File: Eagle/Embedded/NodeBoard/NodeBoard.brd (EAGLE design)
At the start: 121.7 x 96 mm, 68 parts, among them IC1 7812TV, IC2 5v, IC3 3v3, IC4 REG1117, IC5 REG1117, J1 DCJ0202, Q2 IRF740, T1 BC547

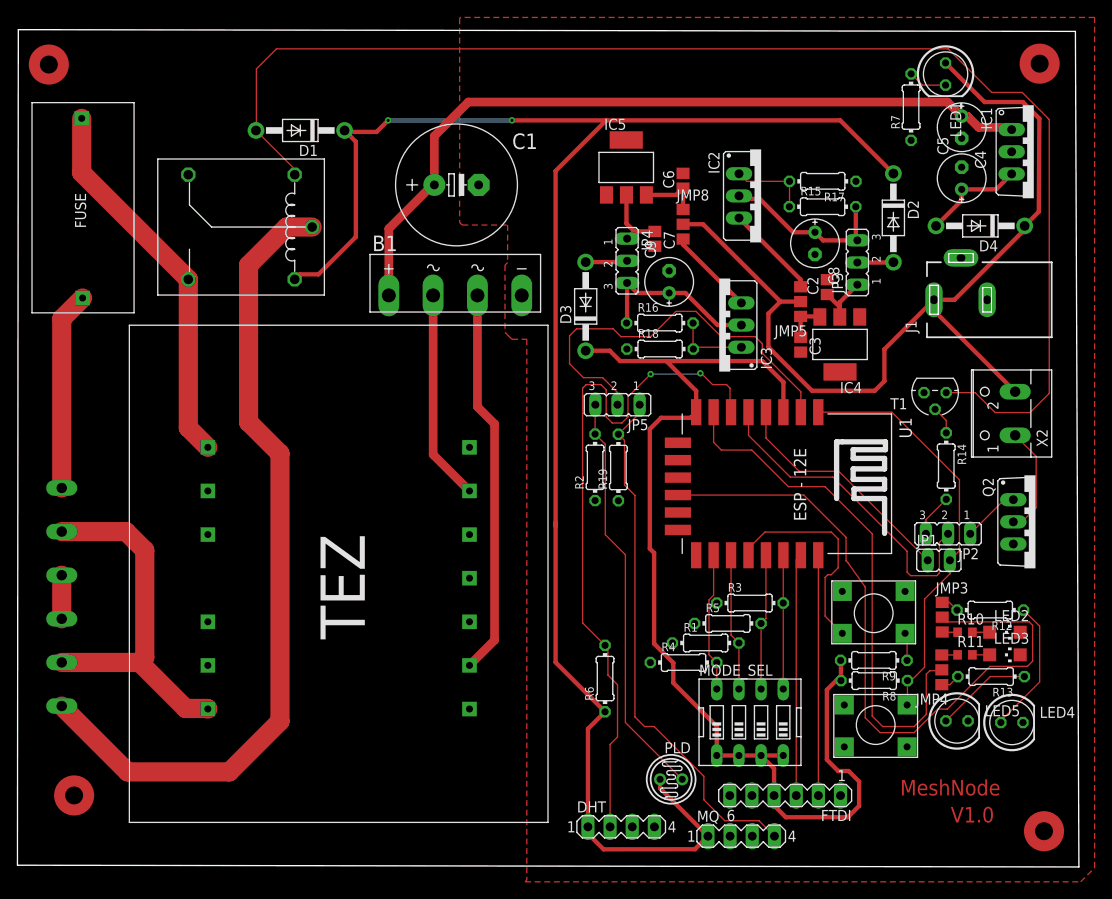
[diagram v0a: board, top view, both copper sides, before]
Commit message: Minor Eagle Board fixes
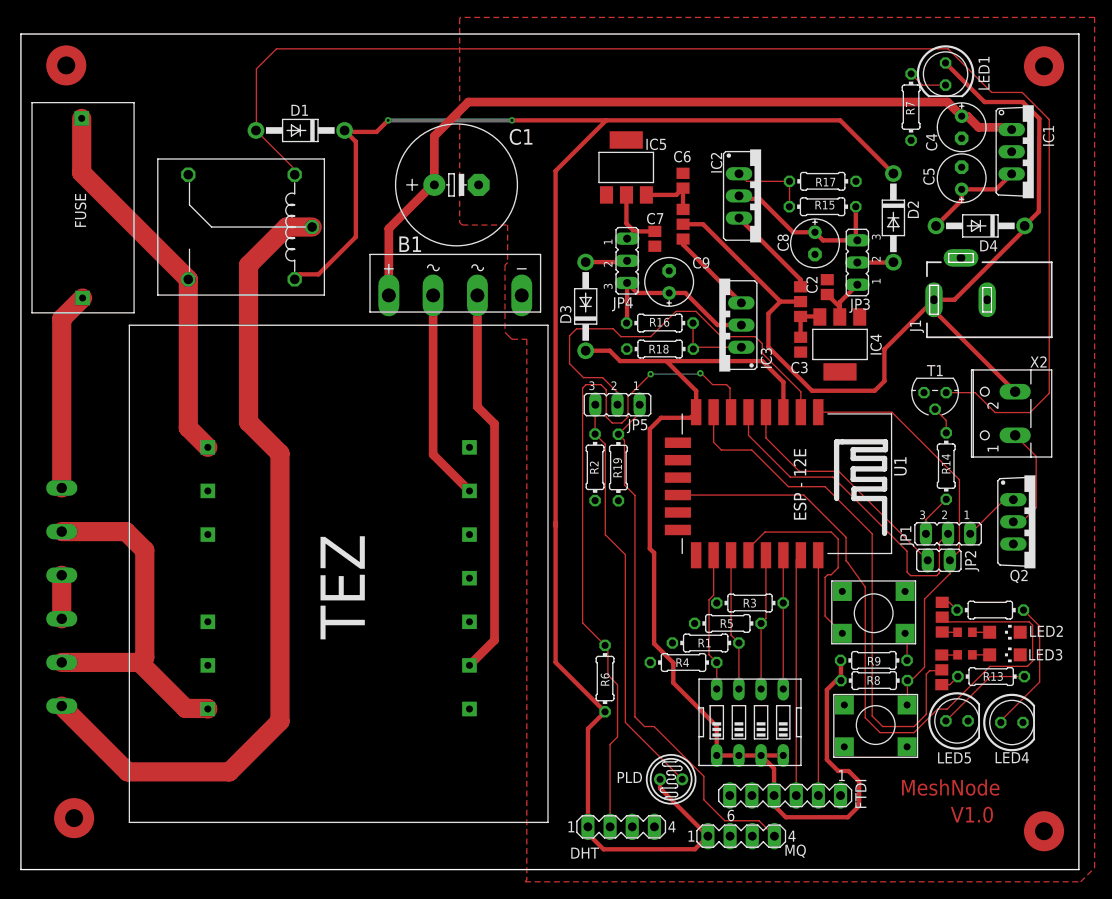
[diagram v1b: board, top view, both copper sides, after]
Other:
- board size 121.7 x 96 mm -> 121.3 x 95.8 mm
